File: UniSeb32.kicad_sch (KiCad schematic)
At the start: 60 parts, among them J1 IO, J101 Micro_SD_Card_Det, J2 ARJM11C7-114-BA-EW2, J3 Conn_02x05_Odd_Even, J6 SDS011, J7 Conn_01x02_Female, J8 Conn_01x02_Female, U1 mini_esp32, U2 LAN8720A, U3 AMS1117-3.3, U4 AMS5915, U5 module_bme280, U6 RT9400, U7 MCP23008-xSS, U8 HLK-PM01, X1 233-508, X2 233-503, X3 233-504

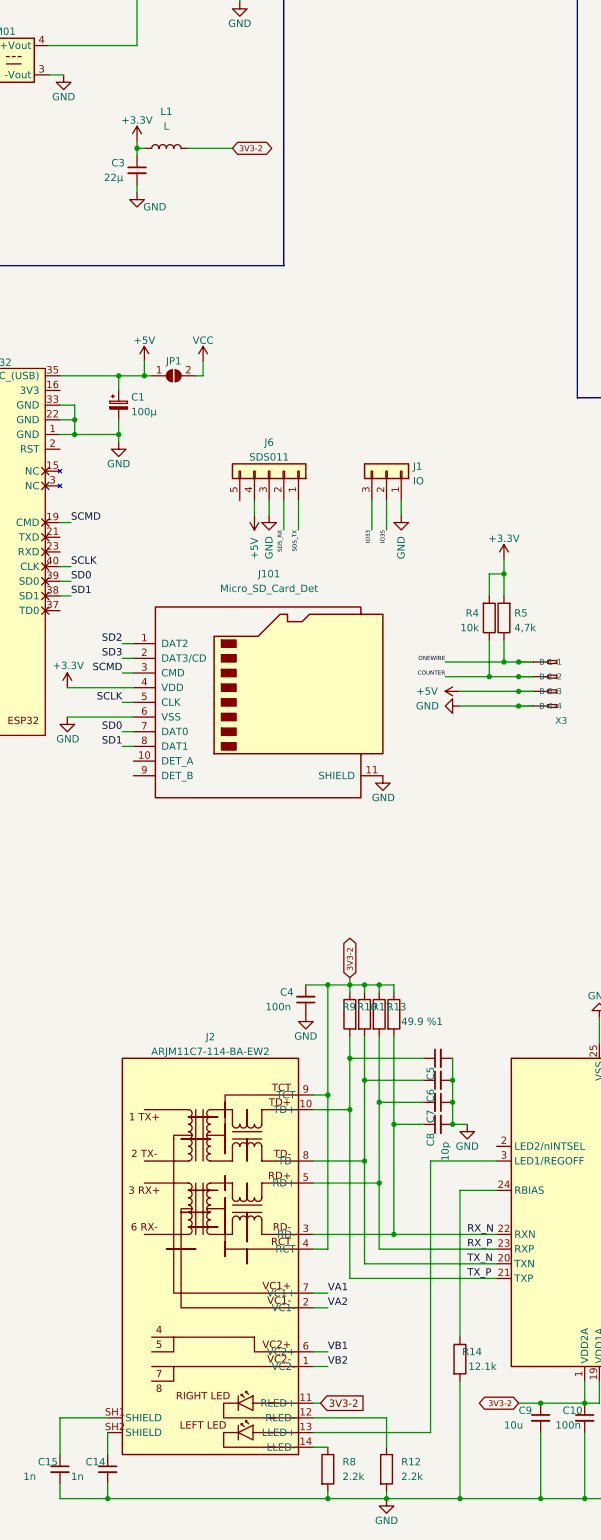
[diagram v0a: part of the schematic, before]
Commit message: .
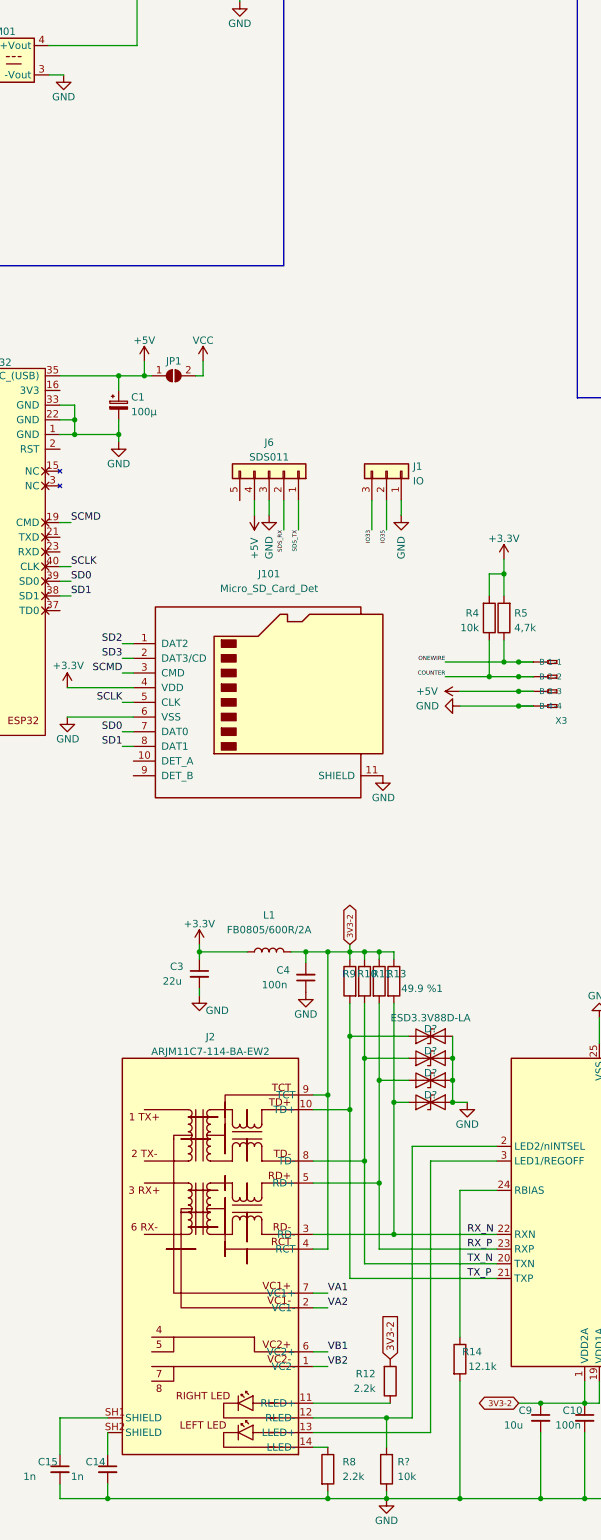
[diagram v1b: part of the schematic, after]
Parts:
- removed C5, C6, C7, C8: 10p, Capacitor_SMD:C_0603_1608Metric, symbol Device:C_Small
- added D? (x4): ESD3.3V88D-LA, Diode_SMD:D_SOD-923, symbol Diode:ESD9B3.3ST5G
- added R?: 10k, Resistor_SMD:R_0603_1608Metric, symbol Device:R
- C3: value 22µ -> 22u
- H3: footprint (none) -> MountingHole:MountingHole_3.2mm_M3
- L1: value L -> FB0805/600R/2A
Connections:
- net 3V3-2: now also R12.2; no longer J2.11 (RLED+)
- net GND: now also D?.2 (A2), D?.2 (A2), D?.2 (A2), D?.2 (A2), R?.1; no longer R12.2
- net RX_N: now also D?.1 (A1)
- net RX_P: now also D?.1 (A1)
- net TX_N: now also D?.1 (A1)
- net TX_P: now also D?.1 (A1)
- net at R12.1: now also J2.11 (RLED+); no longer J2.12 (RLED-)
- net at U2.2 (LED2/nINTSEL): now also J2.12 (RLED-), R?.2
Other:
- moved on the sheet: C3, C4, L1, R10, R11, R12, R13, R9

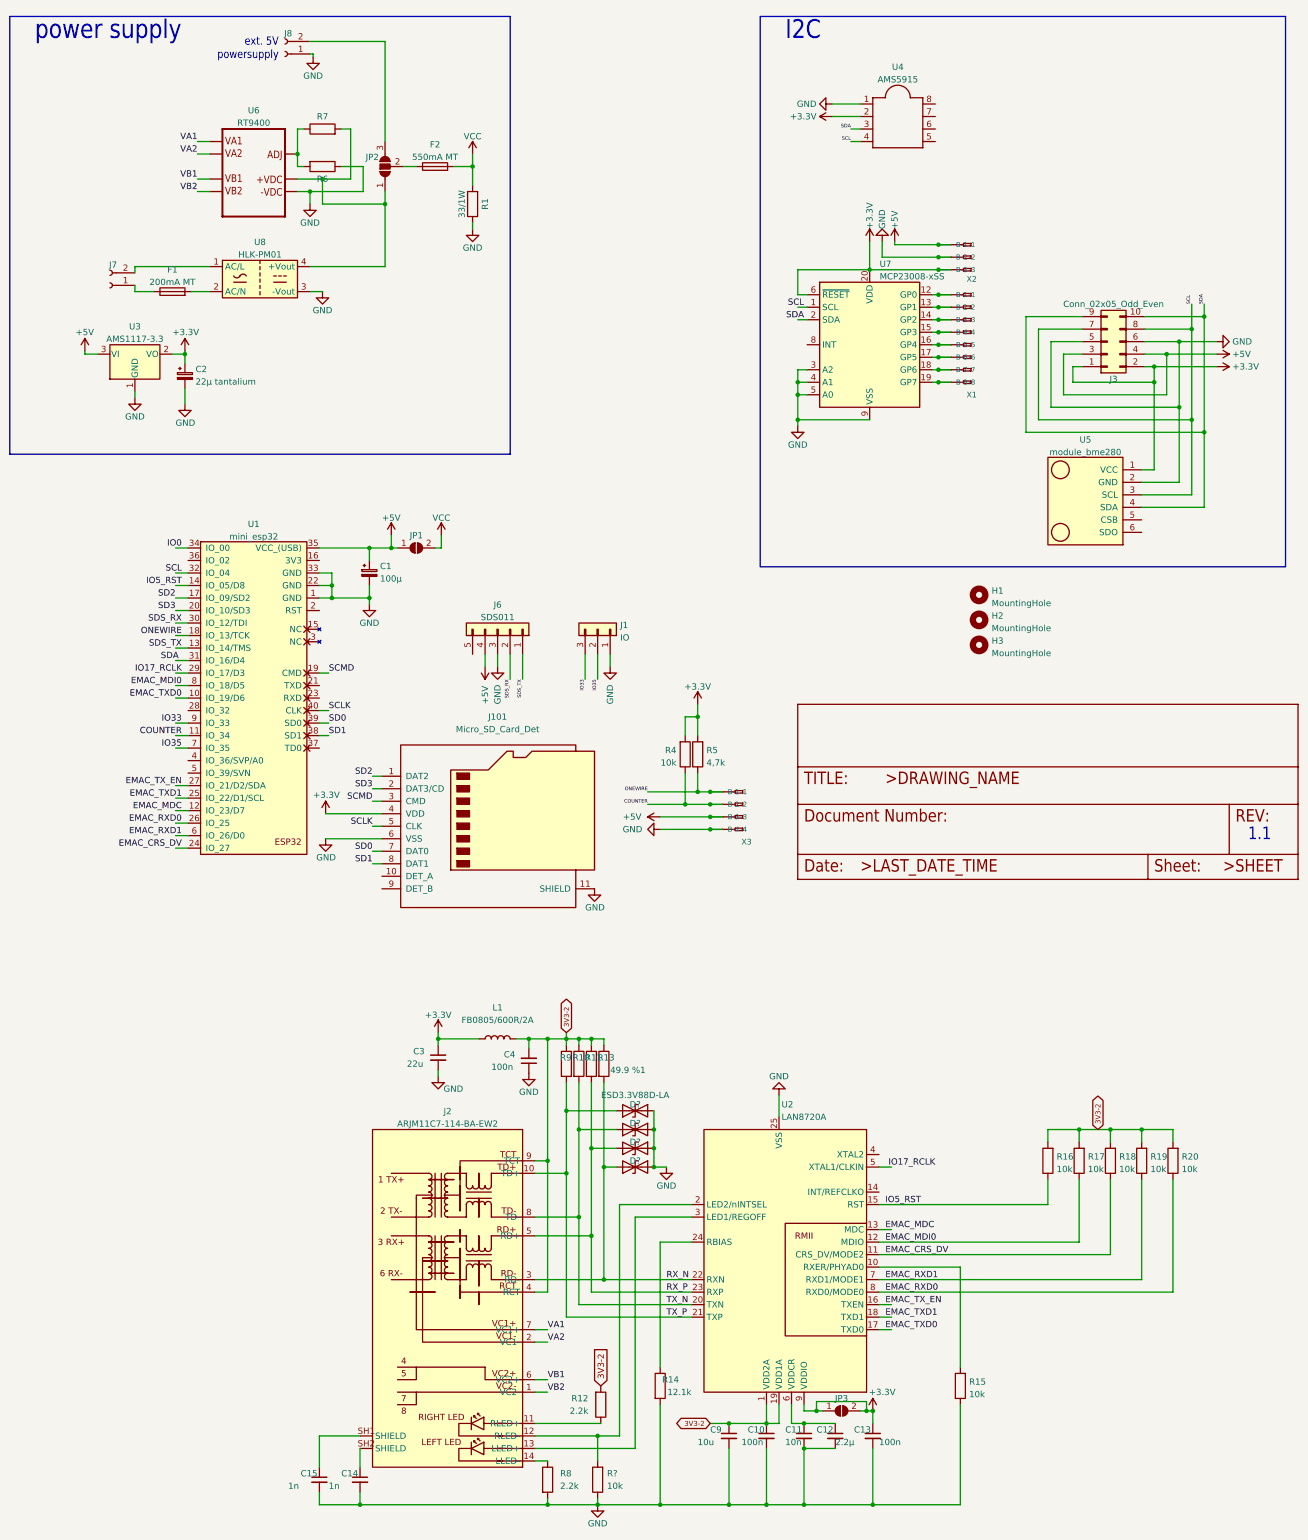
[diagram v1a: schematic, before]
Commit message: .
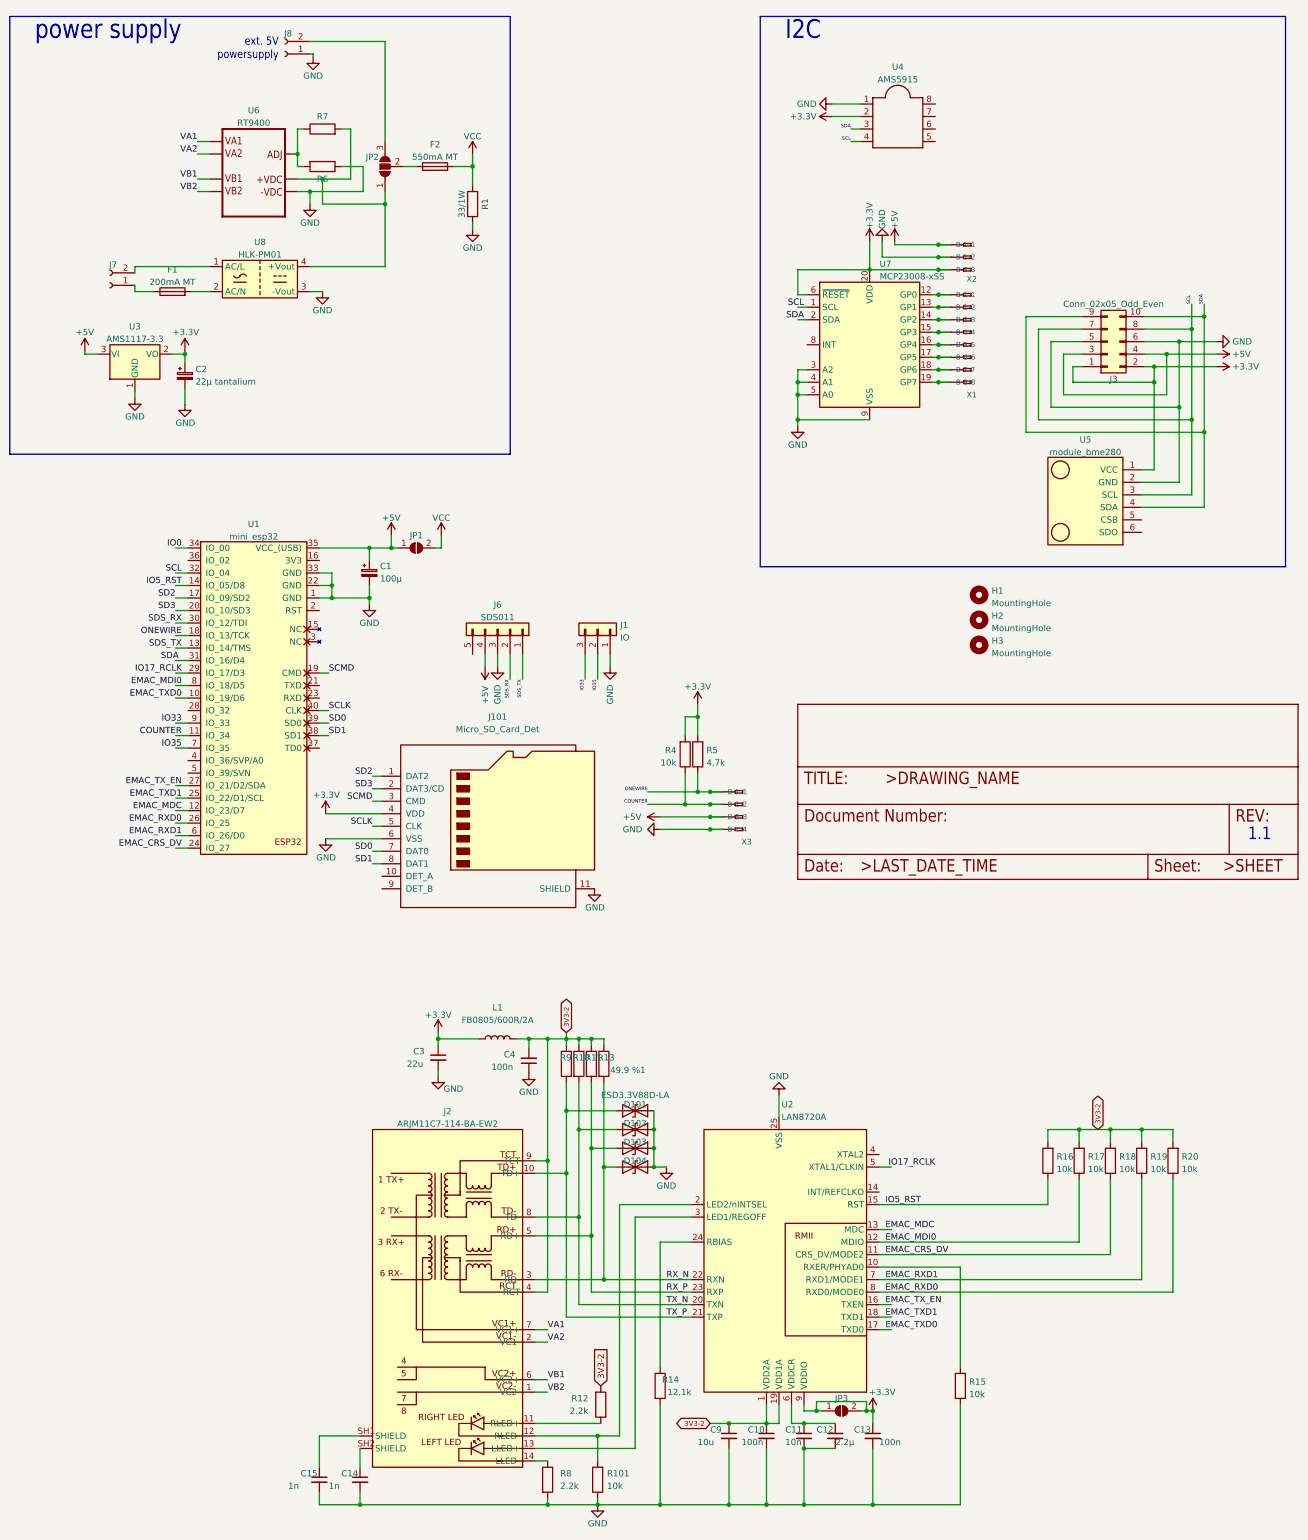
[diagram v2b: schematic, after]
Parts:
- gave numbers to parts that had none: 5
